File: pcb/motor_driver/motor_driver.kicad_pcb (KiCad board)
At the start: 4 copper layers, 55 x 55 mm, 90 parts, among them J1 XT60PW-M, J2 1-84953-1, J3 Conn_ARM_JTAG_SWD_10, J4 UART1 SH, J5 Conn, Q1 BSS138, Q2 HP8K22TB, Q3 HP8K22TB, Q4 HP8K22TB, SW1 RESET, SW2 USER, U1 USBLC6-4SC6, U10 STM32G431CB, U12 MCP2562-E-SN, U3 DRV8323S, U4 a1333, U8 ADP151AUJZ-3.3-R7, U9 NJM12877F33-TE1, Y1 XRCGB16M000FXN02R0

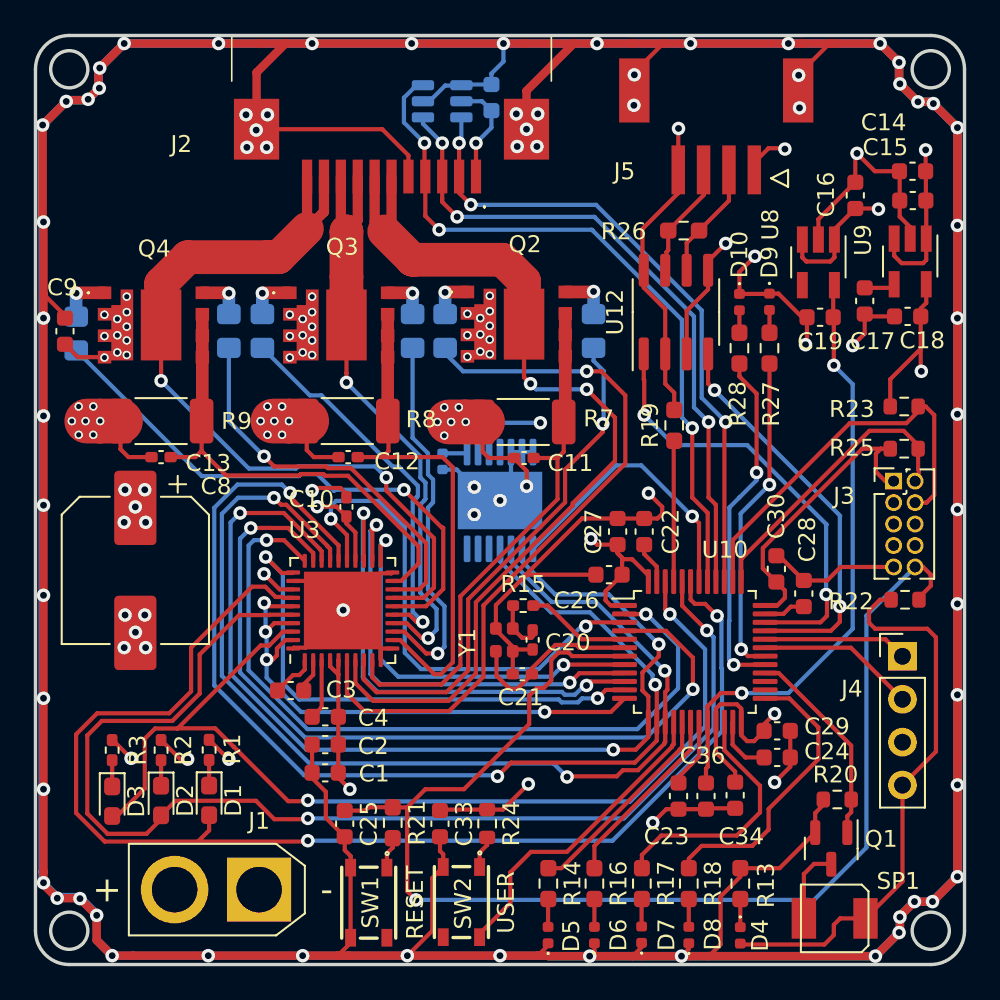
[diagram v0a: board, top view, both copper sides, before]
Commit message: feat: fix most bug
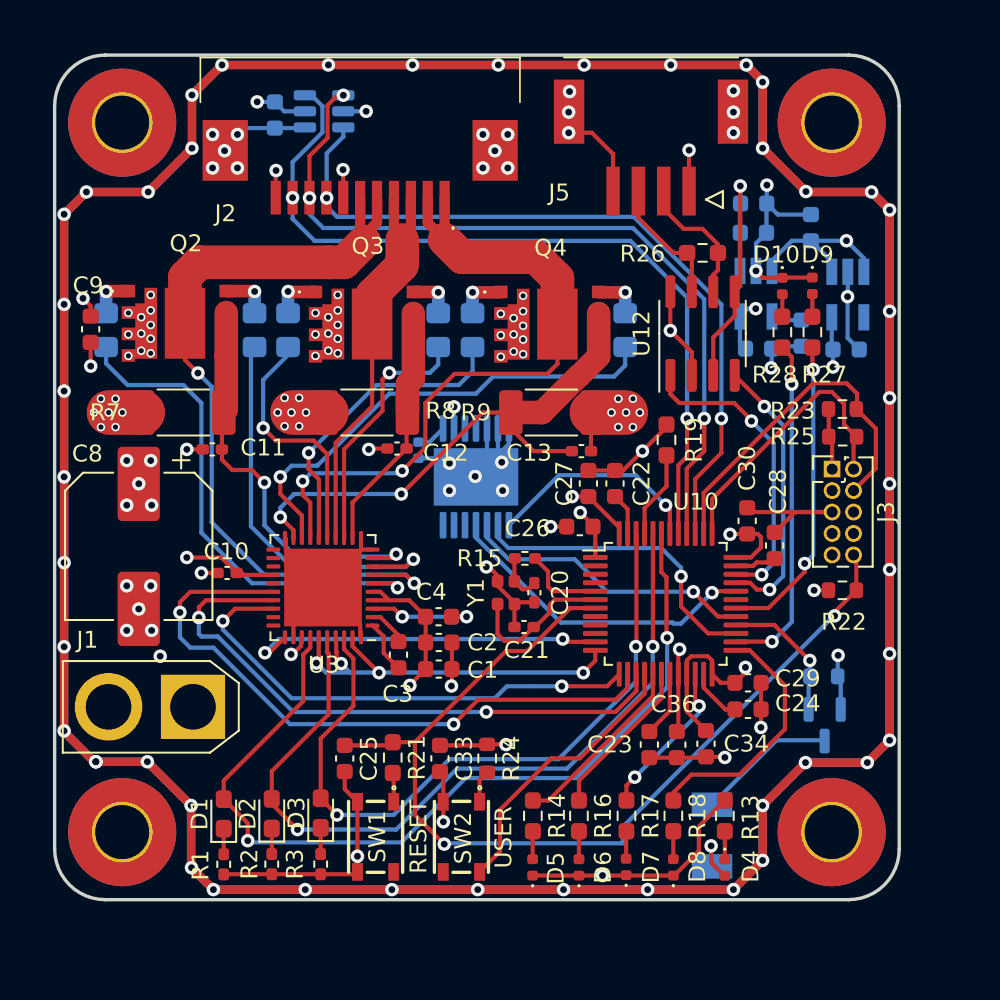
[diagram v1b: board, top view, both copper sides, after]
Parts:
- removed J4: UART1 SH, Connector_PinHeader_2.54mm:PinHeader_1x04_P2.54mm_Vertical
- added H1: MountingHole, MountingHole:MountingHole_3.2mm_M3_Pad_TopBottom, F.Cu at (94.5, 79.3)
- added H2: MountingHole, MountingHole:MountingHole_3.2mm_M3_Pad_TopBottom, F.Cu at (94.5, 121.3)
- added H3: MountingHole, MountingHole:MountingHole_3.2mm_M3_Pad_TopBottom, F.Cu at (136.5, 79.3)
- added H4: MountingHole, MountingHole:MountingHole_3.2mm_M3_Pad_TopBottom, F.Cu at (136.5, 121.3)
- C14, C15, C16, C17, C18, C19, Q1, R20, SP1, U8, U9: moved to B.Cu
- moved C13 24.9 mm to (121.7, 98.8), turned to 0 degrees
- moved R6 23.5 mm to (115.3, 91.6)
- moved Q4 23.5 mm to (119.8, 91.2)
- moved R12 23.5 mm to (124.3, 91.6)
- moved R9 23.1 mm to (119.9, 96.5), turned to 180 degrees
- moved R7 20.1 mm to (98.1, 96.5)
- moved R4 20.1 mm to (93.6, 91.6)
- moved Q2 20.1 mm to (97.8, 91.2)
- moved R10 20.1 mm to (102.4, 91.6)
- moved C11 18.5 mm to (99.9, 98.7)
- moved R3 14.1 mm to (106.3, 123.2), turned to -90 degrees
- moved C5 12.9 mm to (103.6, 78.9), turned to -90 degrees
- moved D3 12.4 mm to (106.3, 120.2), turned to 90 degrees
- moved J1 11.5 mm to (98.7, 113.9)
- moved SP1 9.85 mm to (133.8, 121.3), turned to 90 degrees
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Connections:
- J2 pad 1: +5V -> /drv8323/SHC
- J2 pad 10: /drv8323/SHC -> /drv8323/HALL_W
- J2 pad 11: /drv8323/SHC -> +5V
- J2 pad 2: /drv8323/HALL_W -> /drv8323/SHC
- J2 pad 3: /drv8323/HALL_U -> /drv8323/SHB
- J2 pad 4: /drv8323/HALL_V -> /drv8323/SHB
- J2 pad 5: GND -> /drv8323/SHA
- J2 pad 7: /drv8323/SHA -> GND
- J2 pad 8: /drv8323/SHB -> /drv8323/HALL_V
- J2 pad 9: /drv8323/SHB -> /drv8323/HALL_U
- U10 pad 2: /stm32g431cb/DRV_ENABLE -> /stm32g431cb/FAULTB
- U10 pad 26: unconnected-(U10-Pad26) -> /stm32g431cb/LED_CAN_RX
- U10 pad 27: unconnected-(U10-Pad27) -> /drv8323/SPI2_CLK
- U10 pad 29: /stm32g431cb/LED_CAN_RX -> /drv8323/SPI2_MOSI
- U10 pad 3: /stm32g431cb/FAULTB -> /stm32g431cb/SS_DRV
- U10 pad 31: /stm32g431cb/USART1_TX -> unconnected-(U10-Pad31)
- U10 pad 32: /stm32g431cb/USART1_RX -> /drv8323/SPI2_MISO
- U10 pad 39: /drv8323/HALL_W -> /drv8323/HALL_V
- U10 pad 4: /stm32g431cb/SS_DRV -> /stm32g431cb/DRV_ENABLE
- U10 pad 41: /drv8323/HALL_V -> /drv8323/HALL_W
- U4 pad 10: /drv8323/SPI1_MOSI -> /drv8323/SPI2_MOSI
- U4 pad 11: /drv8323/SPI1_MISO -> /drv8323/SPI2_MISO
- U4 pad 9: /drv8323/SPI1_CLK -> /drv8323/SPI2_CLK
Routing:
- net GND: track 1047.2 -> 875.6 mm, vias 106 -> 113
- net +3.3V: track 89.1 -> 37.6 mm, vias 5 -> 9
- net /stm32g431cb/SS_DRV: track 49.8 -> 0.00 mm, vias 2 -> 0
- net /stm32g431cb/DRV_ENABLE: track 45.7 -> 0.00 mm, vias 2 -> 0
- net /stm32g431cb/FAULTB: track 30.8 -> 0.00 mm, vias 2 -> 0
- net /drv8323/SPI1_CLK: track 59.9 -> 29.5 mm, vias 3 -> 2
- net /drv8323/SPI1_MOSI: track 64.8 -> 35.5 mm, vias 3 -> 2
- net /stm32g431cb/ADC1_3: track 28.9 -> 0.00 mm, vias 2 -> 0
- net /drv8323/SPI1_MISO: track 66.8 -> 38.2 mm, vias 3 -> 2
- net /stm32g431cb/ADC1_2: track 26.8 -> 0.00 mm, vias 2 -> 0
- net /drv8323/INHB: track 71.8 -> 46.9 mm
- net /drv8323/INHA: track 76.4 -> 52.7 mm
- net /stm32g431cb/ADC1_1: track 23.7 -> 0.00 mm, vias 2 -> 0
- net /drv8323/INHC: track 61.4 -> 41.9 mm
- net /drv8323/SPI2_MISO: track 0.00 -> 19.0 mm, vias 0 -> 1
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- removed copper zone on In2.Cu, net GND
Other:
- board size 55 x 55 mm -> 50 x 50 mm
